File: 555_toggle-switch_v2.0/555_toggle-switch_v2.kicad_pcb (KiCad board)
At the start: 2 copper layers, 29.8 x 39.8 mm, 18 parts, among them J1 3V3, J3 OUT, J4 USB-C_Receptacle_PowerOnly_6P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, SW1 SW_Push, SW2 SW_SPDT, SW3 SW_Reed, U1 NE555D, U2 AMS1117-3V3

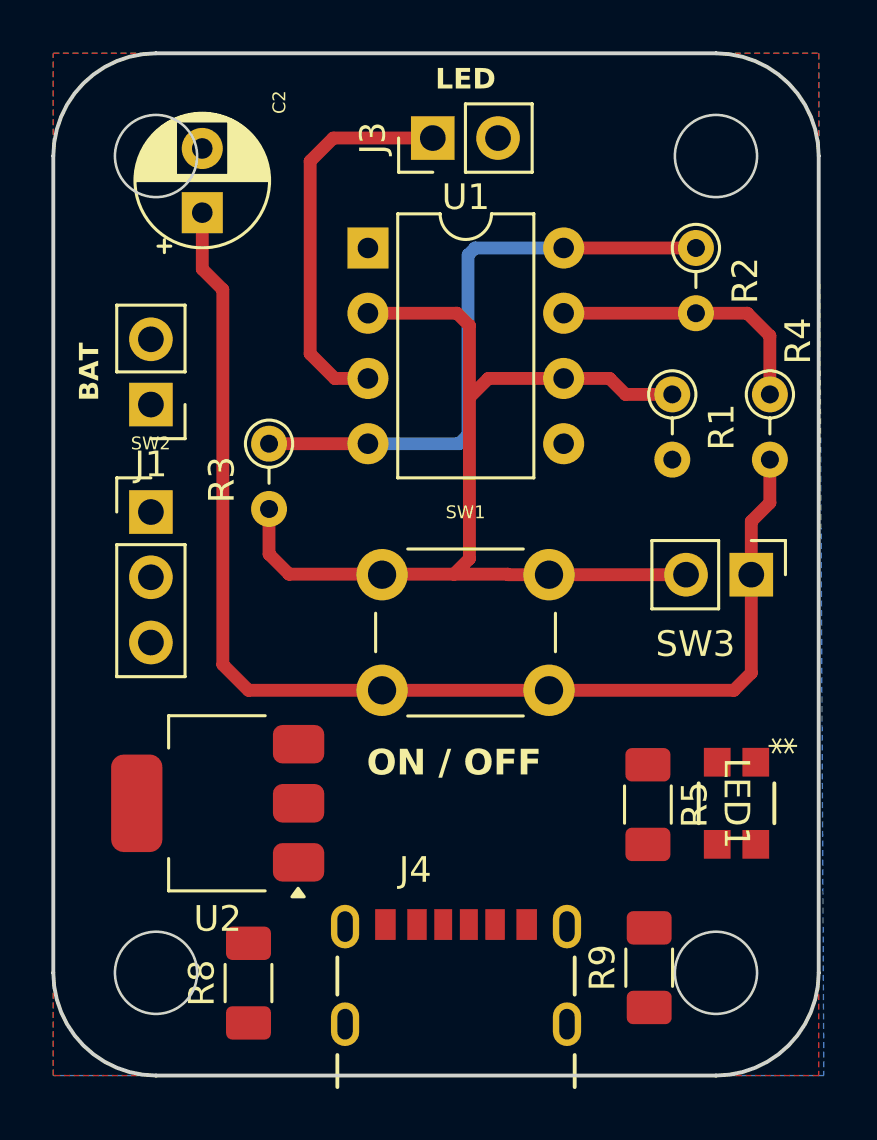
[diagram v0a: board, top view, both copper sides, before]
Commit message: .
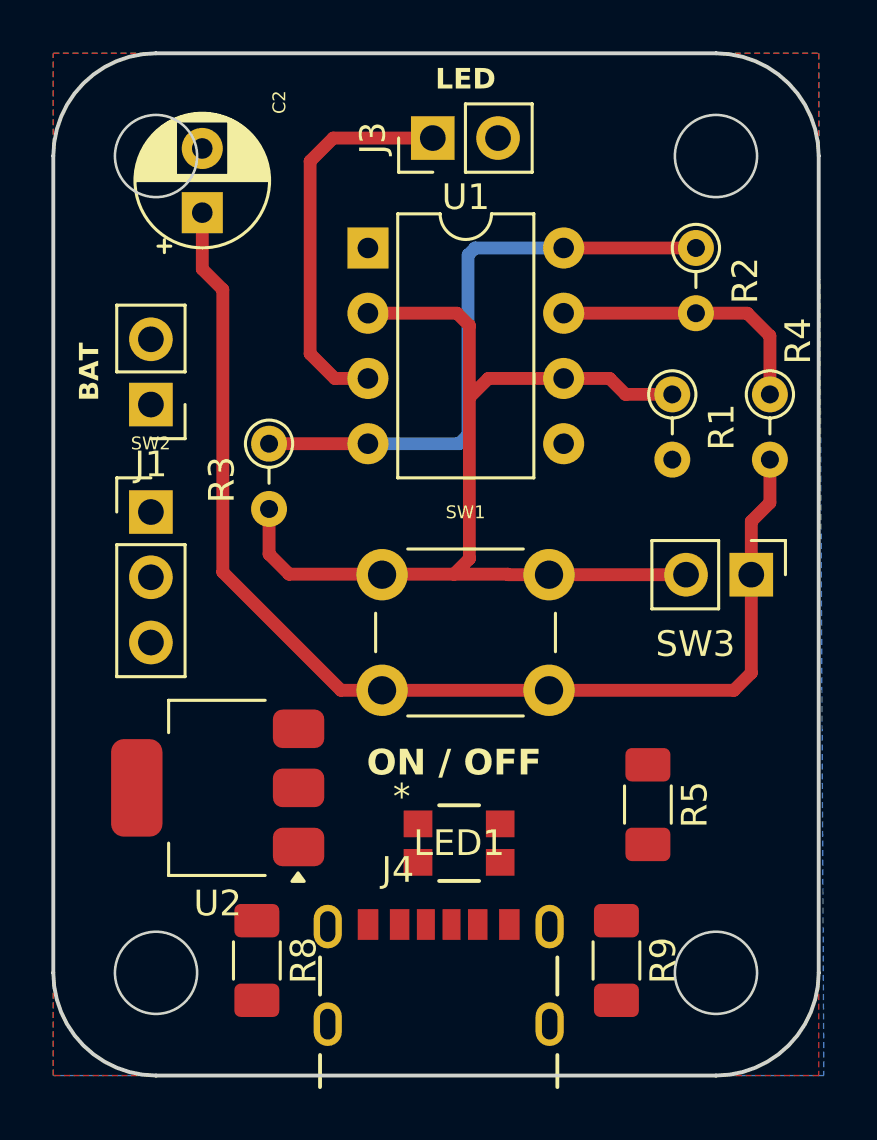
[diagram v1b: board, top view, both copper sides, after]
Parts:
- moved LED1 10.9 mm to (125.4, 117.2), turned to 0 degrees
- moved R9 1.31 mm to (131.5, 121.7), turned to -90 degrees
- moved R8 0.94 mm to (117.5, 121.7), turned to -90 degrees
- moved J4 0.67 mm to (124.6, 126.8)
- moved U2 0.60 mm to (116.0, 115.0)
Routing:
- net Net-(C2-Pad1): track 47.8 -> 45.7 mm
